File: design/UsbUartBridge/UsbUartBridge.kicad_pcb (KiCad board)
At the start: 2 copper layers, 50.9 x 17.8 mm, 15 parts, among them J2 UJ2-MIBH-G-SMT-TR, J3 S2B-PH-SM4-TB_LF__SN_, J4 S2B-PH-SM4-TB_LF__SN_, J5 SM04B-SRSS-TB_LF__SN_, U1 CP2102

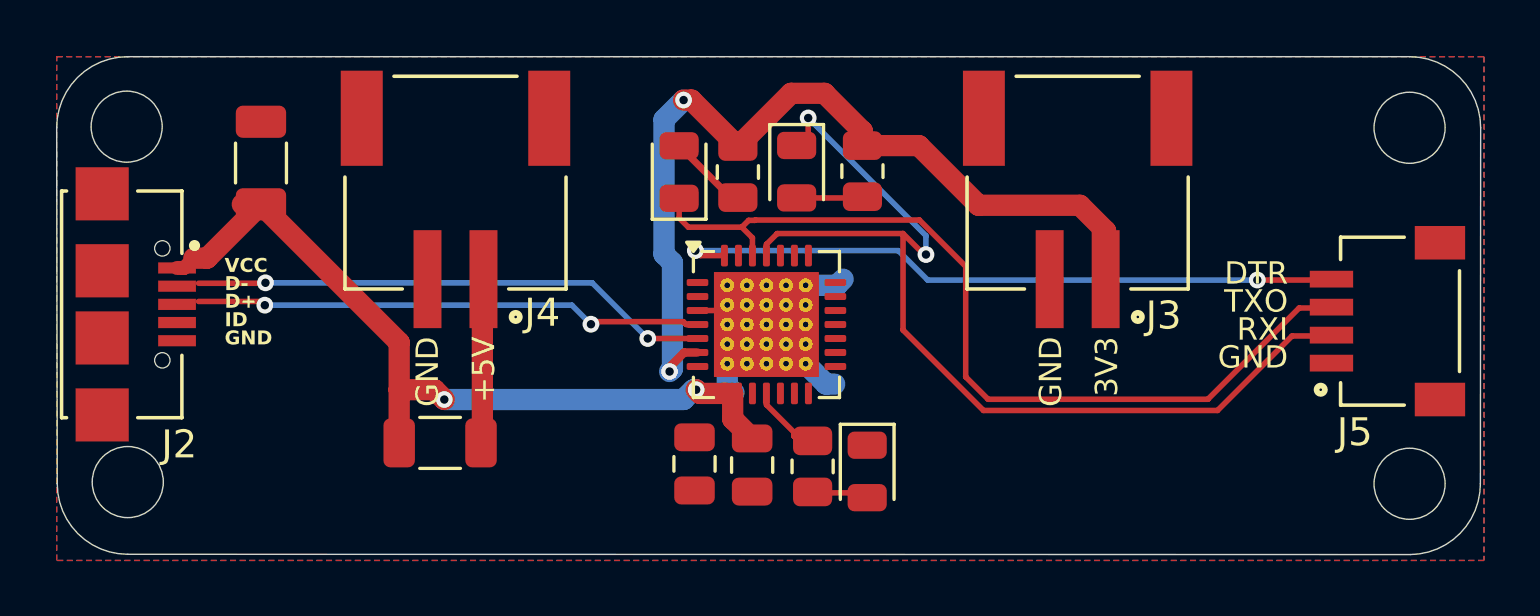
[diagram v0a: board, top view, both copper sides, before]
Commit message: adjustement and gerber files
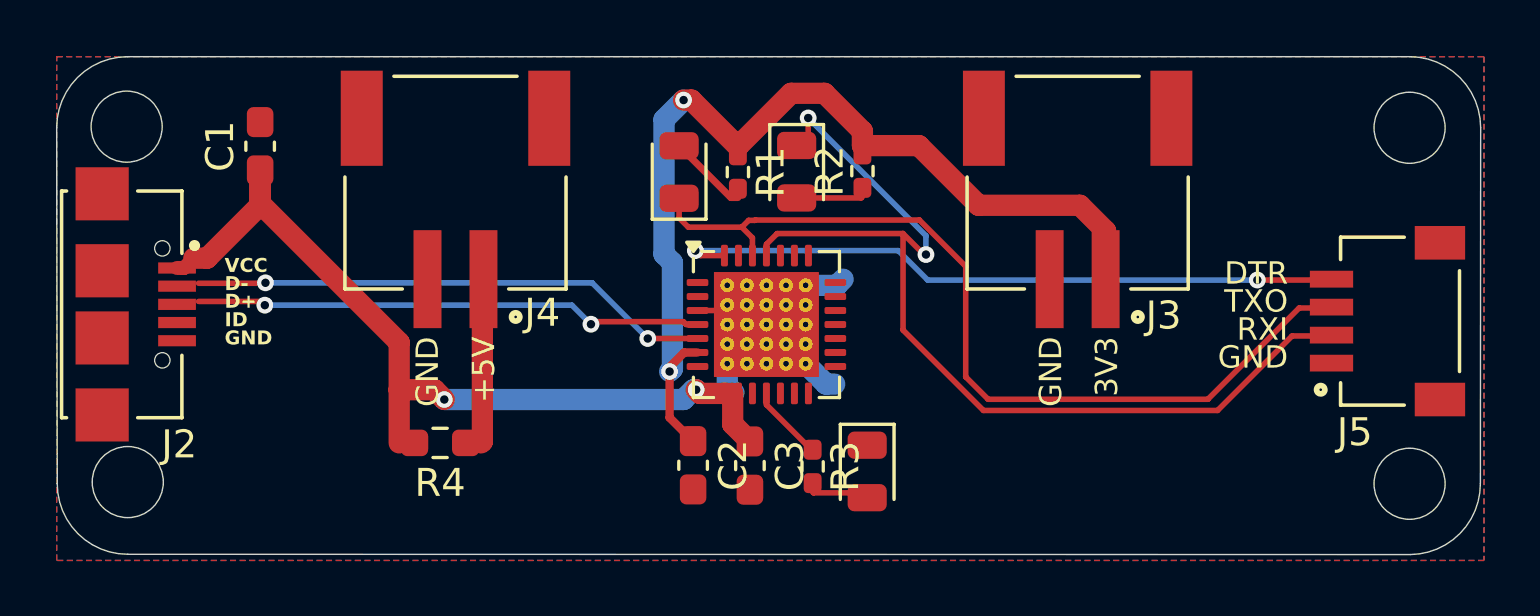
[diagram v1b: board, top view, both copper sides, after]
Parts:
- C1: value C -> 100nF; footprint Capacitor_SMD:C_1206_3216Metric -> Capacitor_SMD:C_0603_1608Metric_Pad1.08x0.95mm_HandSolder
- C2, C3: value C -> 100nF; footprint Capacitor_SMD:C_0805_2012Metric -> Capacitor_SMD:C_0603_1608Metric_Pad1.08x0.95mm_HandSolder
- R1, R2, R3: value R -> 1k; footprint Resistor_SMD:R_0805_2012Metric -> Resistor_SMD:R_0402_1005Metric_Pad0.72x0.64mm_HandSolder
- R4: value R -> 470; footprint Resistor_SMD:R_1206_3216Metric -> Resistor_SMD:R_0603_1608Metric_Pad0.98x0.95mm_HandSolder
- moved C1 0.60 mm to (27.3, 23.2), turned to 90 degrees
- moved C3 0.08 mm to (44.8, 34.6)
- moved C2 0.07 mm to (42.7, 34.6)
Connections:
- C1 pad 1: GND -> VCC
- C1 pad 2: VCC -> GND
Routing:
- net VDD: track 32.2 -> 35.0 mm
- net VCC: track 29.3 -> 31.2 mm
